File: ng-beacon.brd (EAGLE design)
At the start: 70.9 x 76.3 mm, 2 parts

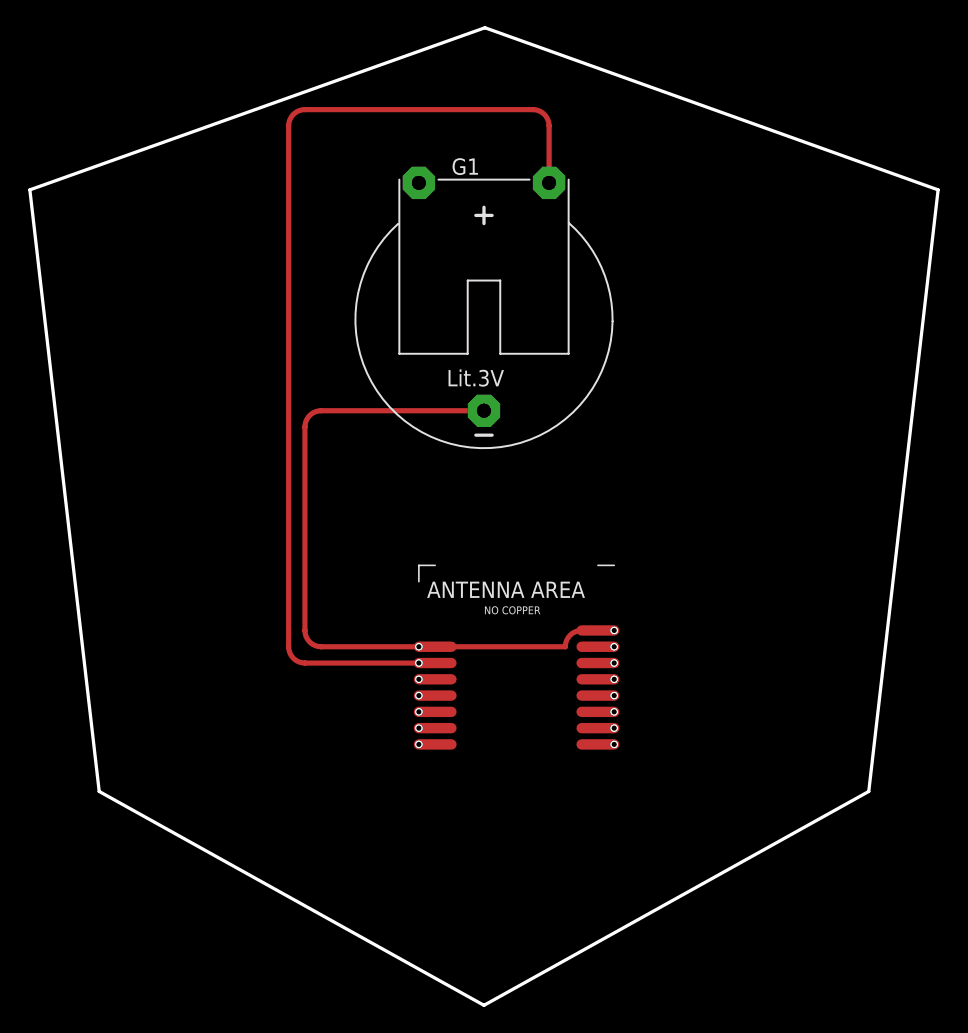
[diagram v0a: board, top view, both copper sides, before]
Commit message: update board layout
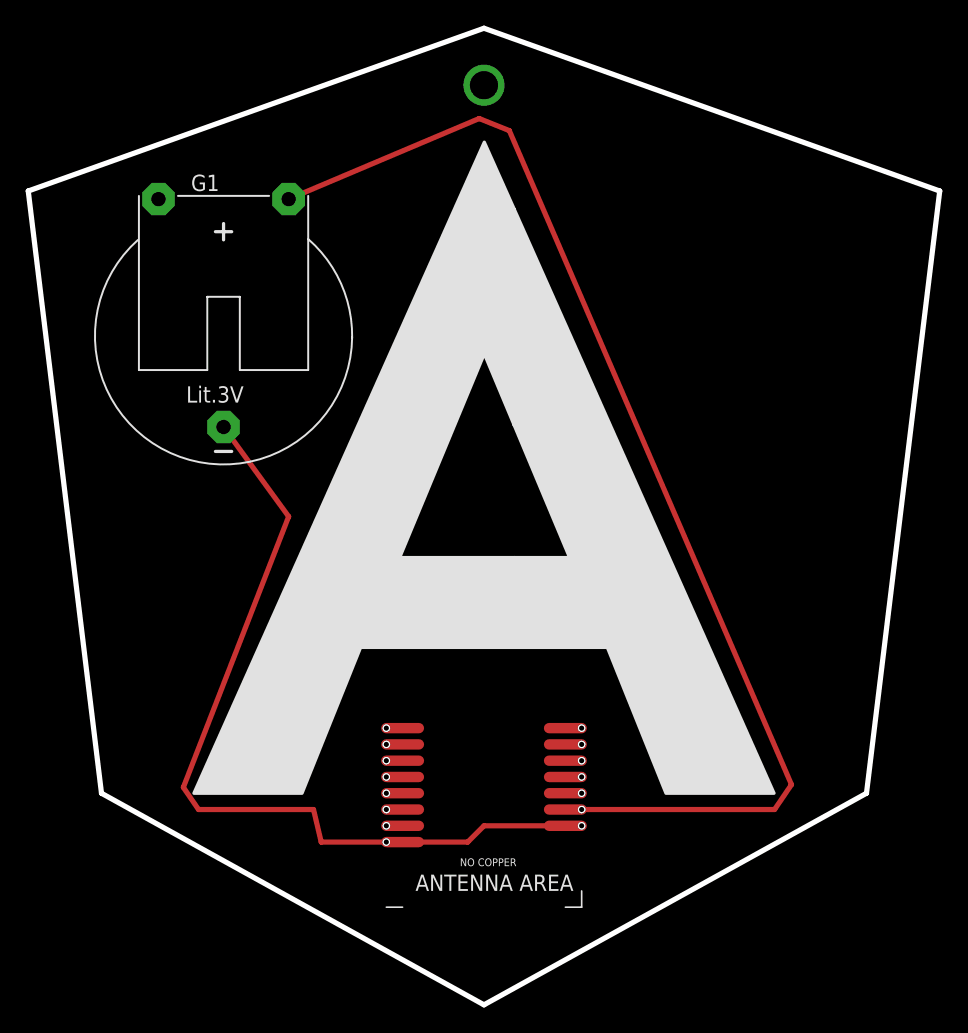
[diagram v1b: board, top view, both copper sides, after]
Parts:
- moved G1 20.4 mm to (25.4, 50.8)
- moved U$1 11.7 mm to (45.7, 14.0), turned to 180 degrees
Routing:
- net N$1: track 78.4 -> 92.9 mm
- net N$2: track 54.3 -> 64.6 mm
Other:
- board size 70.9 x 76.3 mm -> 71.1 x 76.2 mm
- board text removed: "A"
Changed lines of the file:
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@@
 <board>
 <plain>
-<polygon width="0.254" layer="20" spacing="195.58" pour="hatch">
-<vertex x="45.7962" y="74.9681"/>
-<vertex x="10.287" y="62.3189"/>
-<vertex x="15.6972" y="15.3797"/>
-<vertex x="45.72" y="-1.3081"/>
-<vertex x="75.7428" y="15.3797"/>
-<vertex x="81.153" y="62.3189"/>
-</polygon>
-<text x="24.13" y="16.51" size="50.8" layer="26">A</text>
+<polygon width="0.254" layer="26">
+<vertex x="48.0822" y="60.8076"/>
+<vertex x="48.0822" y="43.942"/>
+<vertex x="52.4002" y="33.6296"/>
+<vertex x="48.0822" y="33.6296"/>
+<vertex x="48.0822" y="26.6192"/>
+<vertex x="55.3466" y="26.6192"/>
+<vertex x="59.9186" y="15.24"/>
+<vertex x="68.3514" y="15.24"/>
+</polygon>
+<polygon width="0.254" layer="25">
+<vertex x="48.0822" y="60.8076"/>
+<vertex x="45.7454" y="66.04"/>
+<vertex x="23.0886" y="15.24"/>
+<vertex x="31.5214" y="15.24"/>
+<vertex x="36.0934" y="26.6192"/>
+<vertex x="48.0822" y="26.6192"/>
+<vertex x="48.0822" y="33.6296"/>
+<vertex x="39.1414" y="33.6296"/>
+<vertex x="45.7454" y="49.53"/>
+<vertex x="48.0822" y="43.942"/>
+</polygon>
+<wire x1="10.16" y1="62.23" x2="45.72" y2="74.93" width="0.4064" layer="20"/>
+<wire x1="45.72" y1="74.93" x2="81.28" y2="62.23" width="0.4064" layer="20"/>
+<wire x1="81.28" y1="62.23" x2="75.565" y2="15.24" width="0.4064" layer="20"/>
+<wire x1="75.565" y1="15.24" x2="45.72" y2="-1.27" width="0.4064" layer="20"/>
+<wire x1="45.72" y1="-1.27" x2="15.875" y2="15.24" width="0.4064" layer="20"/>
+<wire x1="15.875" y1="15.24" x2="10.16" y2="62.23" width="0.4064" layer="20"/>
+<polygon width="0.254" layer="25">
+<vertex x="48.0822" y="60.8076"/>
+<vertex x="48.0822" y="43.942"/>
+<vertex x="52.4002" y="33.6296"/>
+<vertex x="48.0822" y="33.6296"/>
+<vertex x="48.0822" y="26.6192"/>
+<vertex x="55.3466" y="26.6192"/>
+<vertex x="59.9186" y="15.24"/>
+<vertex x="68.3514" y="15.24"/>
+</polygon>
+<polygon width="0" layer="27">
+<vertex x="48.0822" y="60.8076"/>
+<vertex x="45.7454" y="66.04"/>
+<vertex x="23.0886" y="15.24"/>
+<vertex x="31.5214" y="15.24"/>
+<vertex x="36.0934" y="26.6192"/>
+<vertex x="48.0822" y="26.6192"/>
+<vertex x="48.0822" y="33.6296"/>
+<vertex x="39.1414" y="33.6296"/>
+<vertex x="45.7454" y="49.53"/>
+<vertex x="48.0822" y="43.942"/>
+</polygon>
+<polygon width="0.254" layer="26">
+<vertex x="48.0822" y="60.8076"/>
+<vertex x="45.7454" y="66.04"/>
+<vertex x="23.0886" y="15.24"/>
+<vertex x="31.5214" y="15.24"/>
+<vertex x="36.0934" y="26.6192"/>
+<vertex x="48.0822" y="26.6192"/>
+<vertex x="48.0822" y="33.6296"/>
+<vertex x="39.1414" y="33.6296"/>
+<vertex x="45.7454" y="49.53"/>
+<vertex x="48.0822" y="43.942"/>
+</polygon>
 </plain>
 <attributes>
@@
 </class>
 </classes>
-<designrules name="default">
+<designrules name="SeeedStudio_2layer_DRU_no_angle_20140221">
 <description language="de">&lt;b&gt;EAGLE Design Rules&lt;/b&gt;
 &lt;p&gt;
@@
 necessary adjustments and save your customized
 design rules under a new name.</description>
+<description language="zh">&lt;b&gt;Seeed Studio EAGLE Design Rules&lt;/b&gt;
+</description>
 <param name="layerSetup" value="(1*16)"/>
-<param name="mtCopper" value="0.035mm 0.035mm 0.035mm 0.035mm 0.035mm 0.035mm 0.035mm 0.035mm 0.035mm 0.035mm 0.035mm 0.035mm 0.035mm 0.035mm 0.035mm 0.035mm"/>
-<param name="mtIsolate" value="1.5mm 0.15mm 0.2mm 0.15mm 0.2mm 0.15mm 0.2mm 0.15mm 0.2mm 0.15mm 0.2mm 0.15mm 0.2mm 0.15mm 0.2mm"/>
-<param name="mdWireWire" value="8mil"/>
-<param name="mdWirePad" value="8mil"/>
-<param name="mdWireVia" value="8mil"/>
-<param name="mdPadPad" value="8mil"/>
-<param name="mdPadVia" value="8mil"/>
-<param name="mdViaVia" value="8mil"/>
-<param name="mdSmdPad" value="8mil"/>
-<param name="mdSmdVia" value="8mil"/>
-<param name="mdSmdSmd" value="8mil"/>
+<param name="mtCopper" value="0.035mm 0.0175mm 0.035mm 0.035mm 0.035mm 0.035mm 0.035mm 0.035mm 0.035mm 0.035mm 0.035mm 0.035mm 0.035mm 0.035mm 0.0175mm 0.035mm"/>
+<param name="mtIsolate" value="1.5mm 1.1mm 0.2mm 0.15mm 0.2mm 0.15mm 0.2mm 0.15mm 0.2mm 0.15mm 0.2mm 0.15mm 0.2mm 0.15mm 0.2mm"/>
+<param name="mdWireWire" value="6mil"/>
+<param name="mdWirePad" value="6mil"/>
+<param name="mdWireVia" value="6mil"/>
+<param name="mdPadPad" value="6mil"/>
+<param name="mdPadVia" value="6mil"/>
+<param name="mdViaVia" value="6mil"/>
+<param name="mdSmdPad" value="0mil"/>
+<param name="mdSmdVia" value="0mil"/>
+<param name="mdSmdSmd" value="0mil"/>
 <param name="mdViaViaSameLayer" value="8mil"/>
 <param name="mnLayersViaInSmd" value="2"/>
-<param name="mdCopperDimension" value="40mil"/>
-<param name="mdDrill" value="8mil"/>
+<param name="mdCopperDimension" value="10mil"/>
+<param name="mdDrill" value="10mil"/>
 <param name="mdSmdStop" value="0mil"/>
-<param name="msWidth" value="10mil"/>
-<param name="msDrill" value="24mil"/>
-<param name="msMicroVia" value="9.99mm"/>
+<param name="msWidth" value="6mil"/>
+<param name="msDrill" value="12mil"/>
+<param name="msMicroVia" value="12mil"/>
 <param name="msBlindViaRatio" value="0.5"/>
 <param name="rvPadTop" value="0.25"/>
@@
 <param name="rlMinPadBottom" value="10mil"/>
 <param name="rlMaxPadBottom" value="20mil"/>
-<param name="rlMinViaOuter" value="8mil"/>
+<param name="rlMinViaOuter" value="6mil"/>
 <param name="rlMaxViaOuter" value="20mil"/>
-<param name="rlMinViaInner" value="8mil"/>
+<param name="rlMinViaInner" value="6mil"/>
 <param name="rlMaxViaInner" value="20mil"/>
 <param name="rlMinMicroViaOuter" value="4mil"/>
@@
 <param name="psTop" value="-1"/>
 <param name="psBottom" value="-1"/>
-<param name="psFirst" value="-1"/>
+<param name="psFirst" value="0"/>
 <param name="psElongationLong" value="100"/>
 <param name="psElongationOffset" value="100"/>
 <param name="mvStopFrame" value="1"/>
 <param name="mvCreamFrame" value="0"/>
-<param name="mlMinStopFrame" value="4mil"/>
-<param name="mlMaxStopFrame" value="4mil"/>
+<param name="mlMinStopFrame" value="2mil"/>
+<param name="mlMaxStopFrame" value="2mil"/>
 <param name="mlMinCreamFrame" value="0mil"/>
 <param name="mlMaxCreamFrame" value="0mil"/>
-<param name="mlViaStopLimit" value="0mil"/>
+<param name="mlViaStopLimit" value="100mil"/>
 <param name="srRoundness" value="0"/>
 <param name="srMinRoundness" value="0mil"/>
@@
 <param name="checkAngle" value="0"/>
 <param name="checkFont" value="1"/>
-<param name="checkRestrict" value="1"/>
+<param name="checkRestrict" value="0"/>
 <param name="useDiameter" value="13"/>
 <param name="maxErrors" value="50"/>
@@
 </autorouter>
 <elements>
-<element name="G1" library="battery" package="CR2032H" value="CR2032H" x="45.72" y="52.07"/>
-<element name="U$1" library="PTR5518" package="PTR5518" value="PTR5518STD" x="48.26" y="25.4"/>
+<element name="G1" library="battery" package="CR2032H" value="CR2032H" x="25.4" y="50.8"/>
+<element name="U$1" library="PTR5518" package="PTR5518" value="PTR5518STD" x="45.72" y="13.97" rot="R180"/>
 </elements>
 <signals>
@@
 <contactref element="G1" pad="+"/>
 <contactref element="U$1" pad="10"/>
-<wire x1="50.8" y1="62.865" x2="50.8" y2="67.31" width="0.4064" layer="1"/>
-<wire x1="50.8" y1="67.31" x2="49.53" y2="68.58" width="0.4064" layer="1" curve="90"/>
-<wire x1="49.53" y1="68.58" x2="31.75" y2="68.58" width="0.4064" layer="1"/>
-<wire x1="31.75" y1="68.58" x2="30.48" y2="67.31" width="0.4064" layer="1" curve="90"/>
-<wire x1="30.48" y1="67.31" x2="30.48" y2="26.67" width="0.4064" layer="1"/>
-<wire x1="30.48" y1="26.67" x2="31.75" y2="25.4" width="0.4064" layer="1" curve="90"/>
-<wire x1="31.75" y1="25.4" x2="41.91" y2="25.4" width="0.4064" layer="1"/>
+<wire x1="52.07" y1="13.97" x2="68.392746875" y2="13.97" width="0.4064" layer="1"/>
+<wire x1="68.392746875" y1="13.97" x2="69.71225625" y2="15.914321875" width="0.4064" layer="1"/>
+<wire x1="69.71225625" y1="15.914321875" x2="47.69648125" y2="66.942515625" width="0.4064" layer="1"/>
+<wire x1="47.69648125" y1="66.942515625" x2="45.347559375" y2="67.885121875" width="0.4064" layer="1"/>
+<wire x1="45.347559375" y1="67.885121875" x2="30.48" y2="61.595" width="0.4064" layer="1"/>
 </signal>
 <signal name="N$2">
@@
 <contactref element="U$1" pad="9"/>
 <contactref element="U$1" pad="8"/>
-<wire x1="45.72" y1="45.085" x2="33.02" y2="45.085" width="0.4064" layer="1"/>
-<wire x1="33.02" y1="45.085" x2="31.75" y2="43.815" width="0.4064" layer="1" curve="90"/>
-<wire x1="31.75" y1="43.815" x2="31.75" y2="27.94" width="0.4064" layer="1"/>
-<wire x1="31.75" y1="27.94" x2="33.02" y2="26.67" width="0.4064" layer="1" curve="90"/>
-<wire x1="33.02" y1="26.67" x2="41.91" y2="26.67" width="0.4064" layer="1"/>
-<wire x1="41.91" y1="26.67" x2="52.07" y2="26.67" width="0.4064" layer="1"/>
-<wire x1="52.07" y1="26.67" x2="53.34" y2="27.94" width="0.4064" layer="1" curve="-90"/>
-<wire x1="53.34" y1="27.94" x2="54.61" y2="27.94" width="0.4064" layer="1"/>
+<wire x1="25.4" y1="43.815" x2="30.48" y2="36.83" width="0.4064" layer="1"/>
+<wire x1="30.48" y1="36.83" x2="22.262896875" y2="15.70030625" width="0.4064" layer="1"/>
+<wire x1="22.262896875" y1="15.70030625" x2="23.44654375" y2="13.97" width="0.4064" layer="1"/>
+<wire x1="23.44654375" y1="13.97" x2="32.4203875" y2="13.97" width="0.4064" layer="1"/>
+<wire x1="32.4203875" y1="13.97" x2="33.02" y2="11.43" width="0.4064" layer="1"/>
+<wire x1="33.02" y1="11.43" x2="39.37" y2="11.43" width="0.4064" layer="1"/>
+<wire x1="39.37" y1="11.43" x2="44.45" y2="11.43" width="0.4064" layer="1"/>
+<wire x1="44.45" y1="11.43" x2="45.72" y2="12.7" width="0.4064" layer="1"/>
+<wire x1="45.72" y1="12.7" x2="52.07" y2="12.7" width="0.4064" layer="1"/>
+</signal>
+<signal name="N$3">
+<via x="45.72" y="70.485" extent="1-16" drill="2.2"/>
 </signal>
 </signals>
